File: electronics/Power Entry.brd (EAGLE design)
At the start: 101.6 x 101.6 mm, 13 parts, among them J1 1-770967-0, J2 1-770969-0, K1 ALQ3F12, P1 703W-00/04

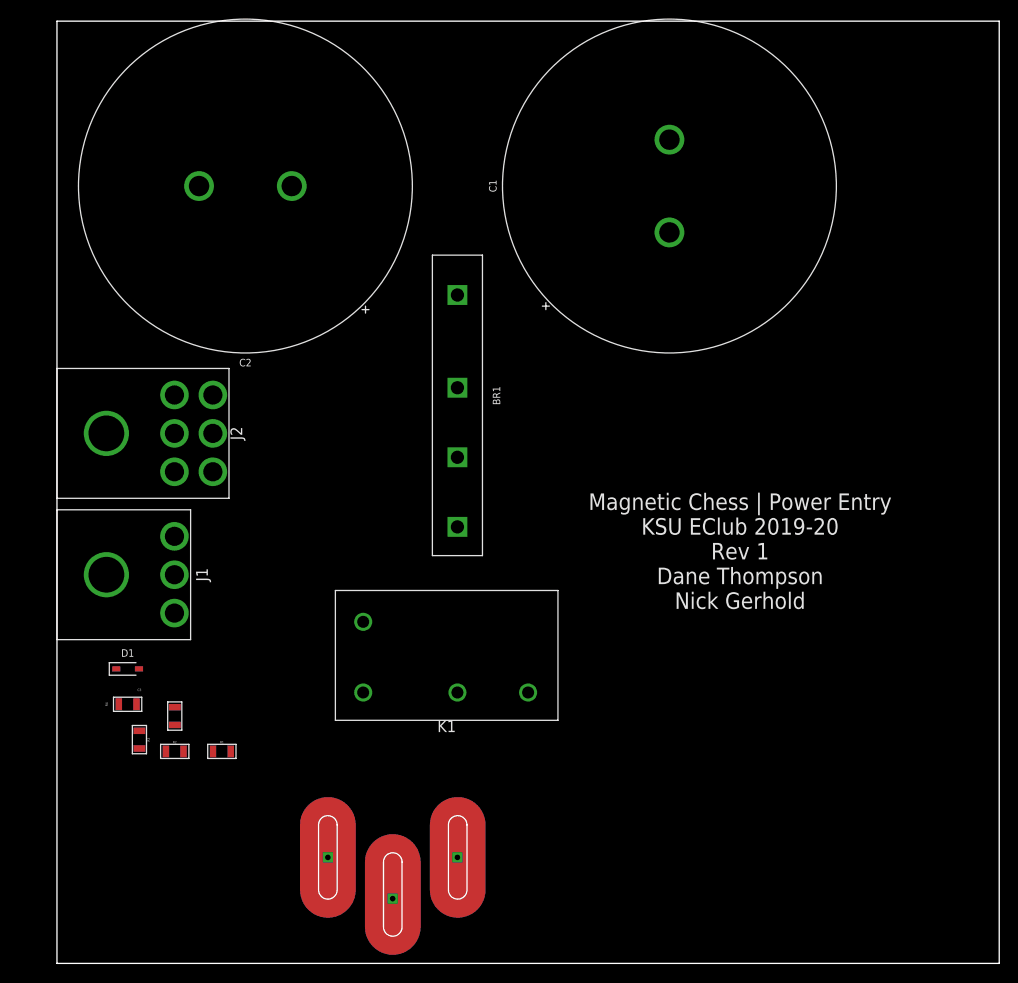
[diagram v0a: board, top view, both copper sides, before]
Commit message: Update Power Entry.brd
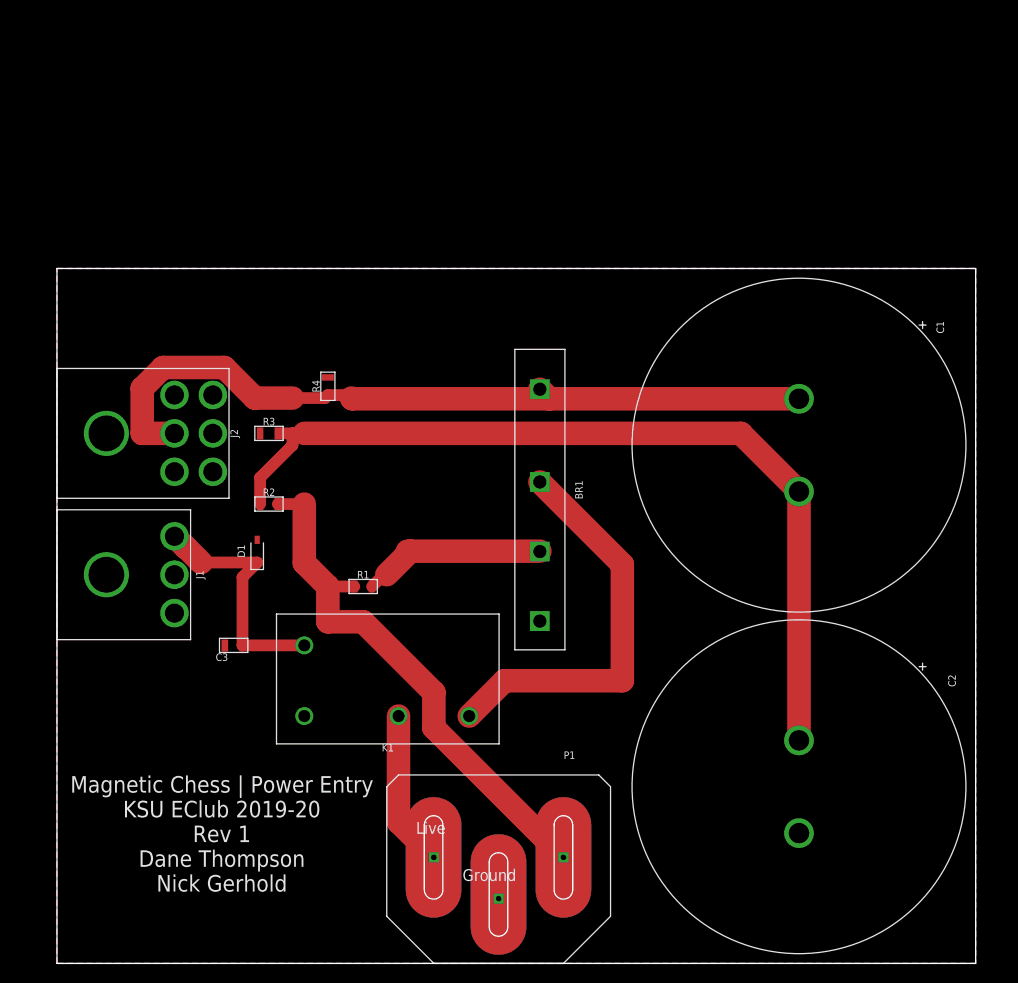
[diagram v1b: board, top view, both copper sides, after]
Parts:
- moved C2 88.1 mm to (80.0, 19.1), turned to 270 degrees
- moved R4 39.2 mm to (29.2, 62.2), turned to 270 degrees
- moved R3 35.9 mm to (22.9, 57.1), turned to 0 degrees
- moved C1 31.2 mm to (80.0, 55.9), turned to 270 degrees
- moved R2 28.5 mm to (22.9, 49.5)
- moved P1 25.4 mm to (54.6, 11.4), flipped to the top
- moved R1 23.4 mm to (33.0, 40.6)
- moved D1 18.9 mm to (21.6, 44.5), turned to 90 degrees
- moved BR1 13.5 mm to (52.1, 41.9)
- moved C3 13.1 mm to (19.1, 34.3), turned to 0 degrees
- moved K1 6.84 mm to (26.7, 26.7)
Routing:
- net N$3: track 0.00 -> 94.4 mm
- net +170V: track 0.00 -> 83.2 mm
- net N$2: track 0.00 -> 57.6 mm
- net N$6: track 0.00 -> 43.2 mm
- net N$8: track 0.00 -> 26.4 mm
- net N$1: track 0.00 -> 20.0 mm
- net N$4: track 0.00 -> 16.8 mm
- added copper zone on layer 1, net GND
- added copper zone on layer 16, net GND
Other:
- board size 101.6 x 101.6 mm -> 99.1 x 74.9 mm
